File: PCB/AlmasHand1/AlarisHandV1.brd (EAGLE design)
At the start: 96.5 x 68.2 mm, 13 parts, among them M1 22-23-2021, M2 22-23-2021, M3 22-23-2021, M4 22-23-2021, M5 22-23-2021, M6 22-23-2021

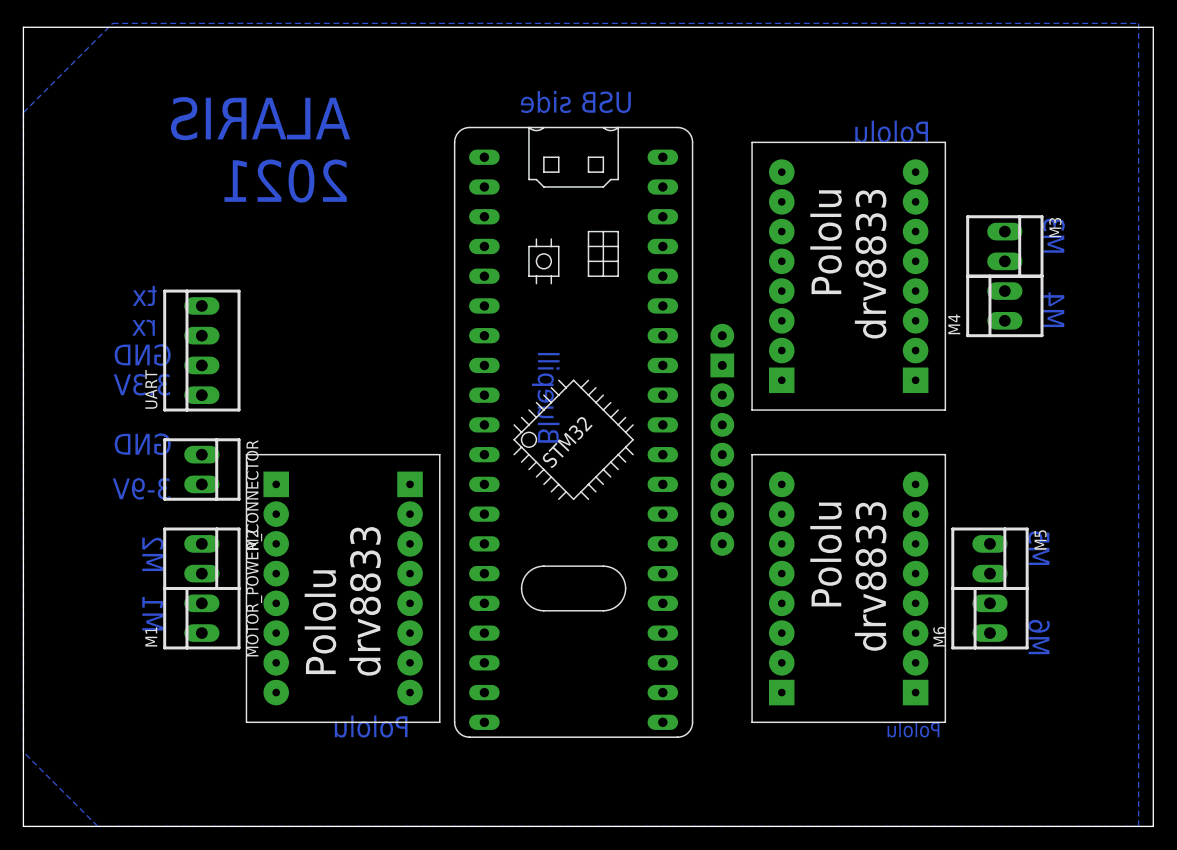
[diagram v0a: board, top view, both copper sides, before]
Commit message: updates on board
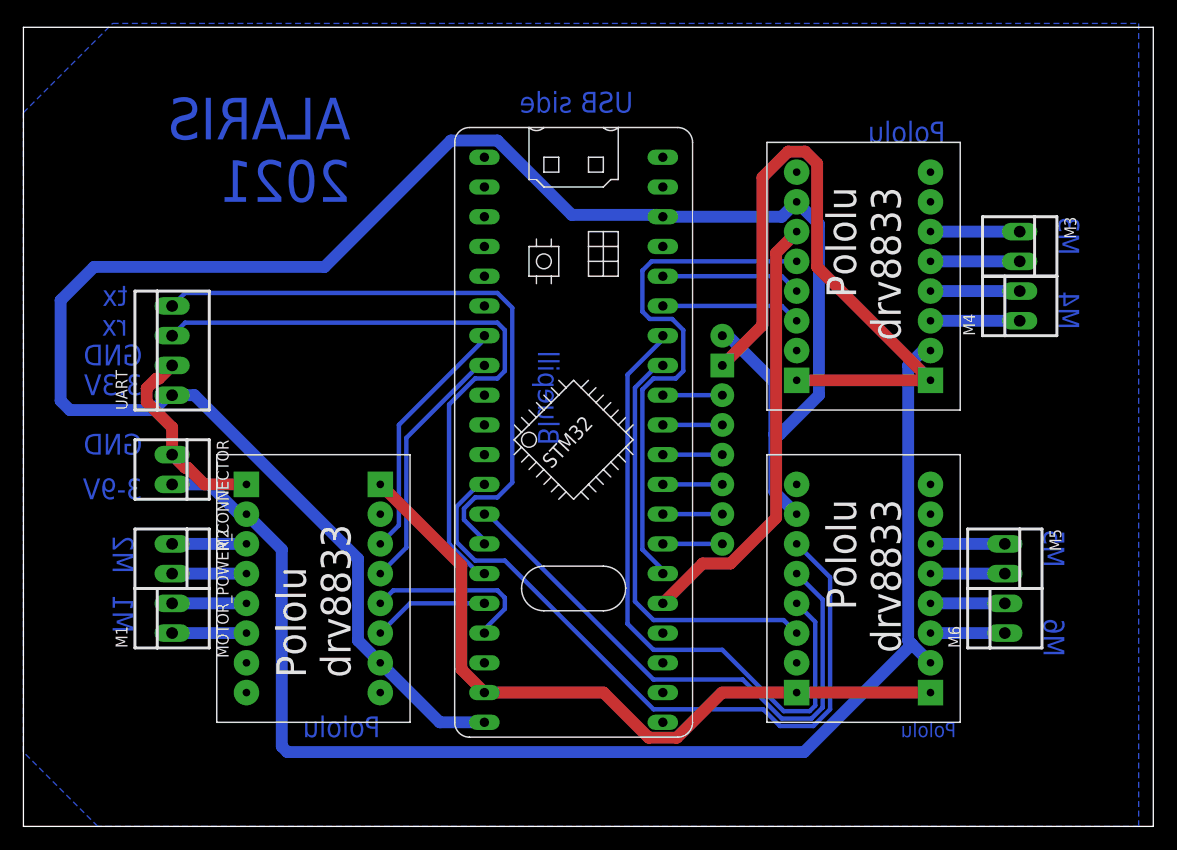
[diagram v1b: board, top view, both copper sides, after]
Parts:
- moved U$1 2.54 mm to (25.4, 14.0)
- moved M1 2.54 mm to (10.2, 15.2)
- moved M2 2.54 mm to (10.2, 20.3)
- moved MOTOR_POWER_CONNECTOR 2.54 mm to (10.2, 27.9)
- moved UART 2.54 mm to (10.2, 38.1)
- moved U$2 1.27 mm to (66.0, 21.6)
- moved U$3 1.27 mm to (66.0, 48.3)
- moved M3 1.27 mm to (82.5, 47.0)
- moved M4 1.27 mm to (82.5, 41.9)
- moved M5 1.27 mm to (81.3, 20.3)
- moved M6 1.27 mm to (81.3, 15.2)
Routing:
- net 3.3V: track 0.00 -> 173.6 mm
- net GND: track 0.00 -> 137.1 mm
- net MOTOR_POWER: track 0.00 -> 114.9 mm
- net N$25: track 0.00 -> 60.5 mm
- net N$32: track 0.00 -> 54.6 mm
- net UART_RX: track 0.00 -> 54.6 mm
- net UART_TX: track 0.00 -> 53.7 mm
- net N$26: track 0.00 -> 48.9 mm
- net N$7: track 0.00 -> 45.2 mm
- net N$8: track 0.00 -> 37.9 mm
- net N$31: track 0.00 -> 36.4 mm
- net N$4: track 0.00 -> 21.7 mm
- net N$3: track 0.00 -> 21.5 mm
- net N$2: track 0.00 -> 15.1 mm
- net N$5: track 0.00 -> 12.0 mm
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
